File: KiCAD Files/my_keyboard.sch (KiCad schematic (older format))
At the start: 47 parts, among them K1 KEYSW, K10 KEYSW, K11 KEYSW, K12 KEYSW, K13 KEYSW, K14 KEYSW, K15 KEYSW, K16 KEYSW, K17 KEYSW, K2 KEYSW, K3 KEYSW, K4 KEYSW, K5 KEYSW, K6 KEYSW, K7 KEYSW, K8 KEYSW, K9 KEYSW, SW1 SW_Push, SW2 Rotary_Encoder_Switch, SW3 Rotary_Encoder_Switch, SW4 Rotary_Encoder_Switch

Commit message: Update PCB
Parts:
- D1, D10, D11, D12, D13, D14, D15, D16, D17, D18, D19, D2, D20, D3, D4, D5, D6, D7, D8, D9: footprint Diode_THT:D_DO-35_SOD27_P10.16mm_Horizontal -> keyboard_parts:D_SOD123_axial
- H1, H2, H3, H4: footprint (none) -> MountingHole:MountingHole_4.3mm_M4_Pad_Via
- SW1: footprint Button_Switch_THT:SW_PUSH_6mm -> Button_Switch_SMD:SW_PUSH_4_5.1x5.1mm
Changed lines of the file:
@@
 F 0 "D1" V 6954 1628 50  0000 L CNN
 F 1 "DIODE" V 7045 1628 50  0000 L CNN
-F 2 "Diode_THT:D_DO-35_SOD27_P10.16mm_Horizontal" H 7000 1500 50  0001 C CNN
+F 2 "keyboard_parts:D_SOD123_axial" H 7000 1500 50  0001 C CNN
 F 3 "~" H 7000 1500 50  0001 C CNN
 	1    7000 1500
@@
 F 0 "D2" V 6954 2478 50  0000 L CNN
 F 1 "DIODE" V 7045 2478 50  0000 L CNN
-F 2 "Diode_THT:D_DO-35_SOD27_P10.16mm_Horizontal" H 7000 2350 50  0001 C CNN
+F 2 "keyboard_parts:D_SOD123_axial" H 7000 2350 50  0001 C CNN
 F 3 "~" H 7000 2350 50  0001 C CNN
 	1    7000 2350
@@
 F 0 "D3" V 6954 3328 50  0000 L CNN
 F 1 "DIODE" V 7045 3328 50  0000 L CNN
-F 2 "Diode_THT:D_DO-35_SOD27_P10.16mm_Horizontal" H 7000 3200 50  0001 C CNN
+F 2 "keyboard_parts:D_SOD123_axial" H 7000 3200 50  0001 C CNN
 F 3 "~" H 7000 3200 50  0001 C CNN
 	1    7000 3200
@@
 F 0 "D4" V 6954 4178 50  0000 L CNN
 F 1 "DIODE" V 7045 4178 50  0000 L CNN
-F 2 "Diode_THT:D_DO-35_SOD27_P10.16mm_Horizontal" H 7000 4050 50  0001 C CNN
+F 2 "keyboard_parts:D_SOD123_axial" H 7000 4050 50  0001 C CNN
 F 3 "~" H 7000 4050 50  0001 C CNN
 	1    7000 4050
@@
 F 0 "D5" V 6954 5028 50  0000 L CNN
 F 1 "DIODE" V 7045 5028 50  0000 L CNN
-F 2 "Diode_THT:D_DO-35_SOD27_P10.16mm_Horizontal" H 7000 4900 50  0001 C CNN
+F 2 "keyboard_parts:D_SOD123_axial" H 7000 4900 50  0001 C CNN
 F 3 "~" H 7000 4900 50  0001 C CNN
 	1    7000 4900
@@
 F 0 "D6" V 7954 1628 50  0000 L CNN
 F 1 "DIODE" V 8045 1628 50  0000 L CNN
-F 2 "Diode_THT:D_DO-35_SOD27_P10.16mm_Horizontal" H 8000 1500 50  0001 C CNN
+F 2 "keyboard_parts:D_SOD123_axial" H 8000 1500 50  0001 C CNN
 F 3 "~" H 8000 1500 50  0001 C CNN
 	1    8000 1500
@@
 F 0 "D7" V 7954 2478 50  0000 L CNN
 F 1 "DIODE" V 8045 2478 50  0000 L CNN
-F 2 "Diode_THT:D_DO-35_SOD27_P10.16mm_Horizontal" H 8000 2350 50  0001 C CNN
+F 2 "keyboard_parts:D_SOD123_axial" H 8000 2350 50  0001 C CNN
 F 3 "~" H 8000 2350 50  0001 C CNN
 	1    8000 2350
@@
 F 0 "D8" V 7954 3328 50  0000 L CNN
 F 1 "DIODE" V 8045 3328 50  0000 L CNN
-F 2 "Diode_THT:D_DO-35_SOD27_P10.16mm_Horizontal" H 8000 3200 50  0001 C CNN
+F 2 "keyboard_parts:D_SOD123_axial" H 8000 3200 50  0001 C CNN
 F 3 "~" H 8000 3200 50  0001 C CNN
 	1    8000 3200
@@
 F 0 "D9" V 7954 4178 50  0000 L CNN
 F 1 "DIODE" V 8045 4178 50  0000 L CNN
-F 2 "Diode_THT:D_DO-35_SOD27_P10.16mm_Horizontal" H 8000 4050 50  0001 C CNN
+F 2 "keyboard_parts:D_SOD123_axial" H 8000 4050 50  0001 C CNN
 F 3 "~" H 8000 4050 50  0001 C CNN
 	1    8000 4050
@@
 F 0 "D10" V 7954 5028 50  0000 L CNN
 F 1 "DIODE" V 8045 5028 50  0000 L CNN
-F 2 "Diode_THT:D_DO-35_SOD27_P10.16mm_Horizontal" H 8000 4900 50  0001 C CNN
+F 2 "keyboard_parts:D_SOD123_axial" H 8000 4900 50  0001 C CNN
 F 3 "~" H 8000 4900 50  0001 C CNN
 	1    8000 4900
@@
 F 0 "D11" V 8954 1628 50  0000 L CNN
 F 1 "DIODE" V 9045 1628 50  0000 L CNN
-F 2 "Diode_THT:D_DO-35_SOD27_P10.16mm_Horizontal" H 9000 1500 50  0001 C CNN
+F 2 "keyboard_parts:D_SOD123_axial" H 9000 1500 50  0001 C CNN
 F 3 "~" H 9000 1500 50  0001 C CNN
 	1    9000 1500
@@
 F 0 "D12" V 8954 2478 50  0000 L CNN
 F 1 "DIODE" V 9045 2478 50  0000 L CNN
-F 2 "Diode_THT:D_DO-35_SOD27_P10.16mm_Horizontal" H 9000 2350 50  0001 C CNN
+F 2 "keyboard_parts:D_SOD123_axial" H 9000 2350 50  0001 C CNN
 F 3 "~" H 9000 2350 50  0001 C CNN
 	1    9000 2350
@@
 F 0 "D13" V 8954 3328 50  0000 L CNN
 F 1 "DIODE" V 9045 3328 50  0000 L CNN
-F 2 "Diode_THT:D_DO-35_SOD27_P10.16mm_Horizontal" H 9000 3200 50  0001 C CNN
+F 2 "keyboard_parts:D_SOD123_axial" H 9000 3200 50  0001 C CNN
 F 3 "~" H 9000 3200 50  0001 C CNN
 	1    9000 3200
@@
 F 0 "D14" V 8954 4178 50  0000 L CNN
 F 1 "DIODE" V 9045 4178 50  0000 L CNN
-F 2 "Diode_THT:D_DO-35_SOD27_P10.16mm_Horizontal" H 9000 4050 50  0001 C CNN
+F 2 "keyboard_parts:D_SOD123_axial" H 9000 4050 50  0001 C CNN
 F 3 "~" H 9000 4050 50  0001 C CNN
 	1    9000 4050
@@
 F 0 "D18" V 9954 3328 50  0000 L CNN
 F 1 "DIODE" V 10045 3328 50  0000 L CNN
-F 2 "Diode_THT:D_DO-35_SOD27_P10.16mm_Horizontal" H 10000 3200 50  0001 C CNN
+F 2 "keyboard_parts:D_SOD123_axial" H 10000 3200 50  0001 C CNN
 F 3 "~" H 10000 3200 50  0001 C CNN
 	1    10000 3200
@@
 F 0 "D16" V 9954 1628 50  0000 L CNN
 F 1 "DIODE" V 10045 1628 50  0000 L CNN
-F 2 "Diode_THT:D_DO-35_SOD27_P10.16mm_Horizontal" H 10000 1500 50  0001 C CNN
+F 2 "keyboard_parts:D_SOD123_axial" H 10000 1500 50  0001 C CNN
 F 3 "~" H 10000 1500 50  0001 C CNN
 	1    10000 1500
@@
 F 0 "D17" V 9954 2478 50  0000 L CNN
 F 1 "DIODE" V 10045 2478 50  0000 L CNN
-F 2 "Diode_THT:D_DO-35_SOD27_P10.16mm_Horizontal" H 10000 2350 50  0001 C CNN
+F 2 "keyboard_parts:D_SOD123_axial" H 10000 2350 50  0001 C CNN
 F 3 "~" H 10000 2350 50  0001 C CNN
 	1    10000 2350
@@
 F 0 "D19" V 9954 4178 50  0000 L CNN
 F 1 "DIODE" V 10045 4178 50  0000 L CNN
-F 2 "Diode_THT:D_DO-35_SOD27_P10.16mm_Horizontal" H 10000 4050 50  0001 C CNN
+F 2 "keyboard_parts:D_SOD123_axial" H 10000 4050 50  0001 C CNN
 F 3 "~" H 10000 4050 50  0001 C CNN
 	1    10000 4050
@@
 F 0 "SW1" H 1300 6835 50  0000 C CNN
 F 1 "SW_Push" H 1300 6744 50  0000 C CNN
-F 2 "Button_Switch_THT:SW_PUSH_6mm" H 1300 6750 50  0001 C CNN
+F 2 "Button_Switch_SMD:SW_PUSH_4_5.1x5.1mm" H 1300 6750 50  0001 C CNN
 F 3 "~" H 1300 6750 50  0001 C CNN
 	1    1300 6550
@@
 F 0 "D15" V 8954 5028 50  0000 L CNN
 F 1 "DIODE" V 9045 5028 50  0000 L CNN
-F 2 "Diode_THT:D_DO-35_SOD27_P10.16mm_Horizontal" H 9000 4900 50  0001 C CNN
+F 2 "keyboard_parts:D_SOD123_axial" H 9000 4900 50  0001 C CNN
 F 3 "~" H 9000 4900 50  0001 C CNN
 	1    9000 4900
@@
 F 0 "D20" V 9954 5028 50  0000 L CNN
 F 1 "DIODE" V 10045 5028 50  0000 L CNN
-F 2 "Diode_THT:D_DO-35_SOD27_P10.16mm_Horizontal" H 10000 4900 50  0001 C CNN
+F 2 "keyboard_parts:D_SOD123_axial" H 10000 4900 50  0001 C CNN
 F 3 "~" H 10000 4900 50  0001 C CNN
 	1    10000 4900
@@
 F 0 "H1" V 4604 4150 50  0000 L CNN
 F 1 "MountingHole_Pad" V 4695 4150 50  0000 L CNN
-F 2 "" H 4650 4000 50  0001 C CNN
+F 2 "MountingHole:MountingHole_4.3mm_M4_Pad_Via" H 4650 4000 50  0001 C CNN
 F 3 "~" H 4650 4000 50  0001 C CNN
 	1    4650 4000
@@
 F 0 "H2" V 4604 4450 50  0000 L CNN
 F 1 "MountingHole_Pad" V 4695 4450 50  0000 L CNN
-F 2 "" H 4650 4300 50  0001 C CNN
+F 2 "MountingHole:MountingHole_4.3mm_M4_Pad_Via" H 4650 4300 50  0001 C CNN
 F 3 "~" H 4650 4300 50  0001 C CNN
 	1    4650 4300
@@
 F 0 "H3" V 4604 4750 50  0000 L CNN
 F 1 "MountingHole_Pad" V 4695 4750 50  0000 L CNN
-F 2 "" H 4650 4600 50  0001 C CNN
+F 2 "MountingHole:MountingHole_4.3mm_M4_Pad_Via" H 4650 4600 50  0001 C CNN
 F 3 "~" H 4650 4600 50  0001 C CNN
 	1    4650 4600
@@
 F 0 "H4" V 4604 5050 50  0000 L CNN
 F 1 "MountingHole_Pad" V 4695 5050 50  0000 L CNN
-F 2 "" H 4650 4900 50  0001 C CNN
+F 2 "MountingHole:MountingHole_4.3mm_M4_Pad_Via" H 4650 4900 50  0001 C CNN
 F 3 "~" H 4650 4900 50  0001 C CNN
 	1    4650 4900

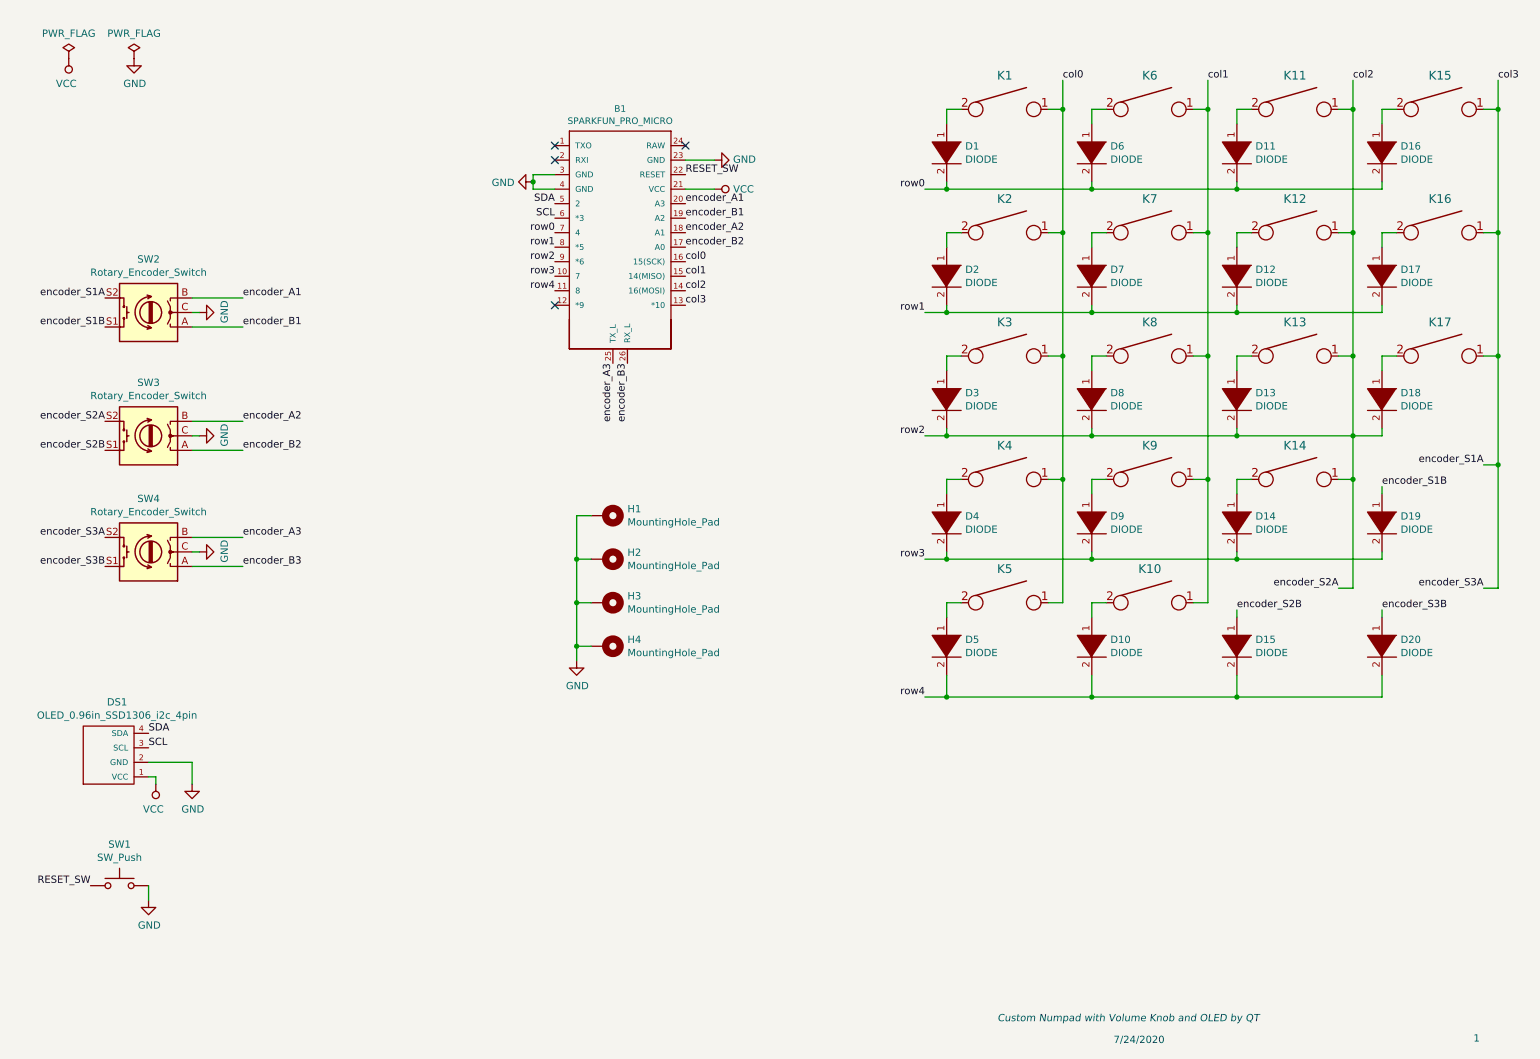
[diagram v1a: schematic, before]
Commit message: Updated KiCAD Schem
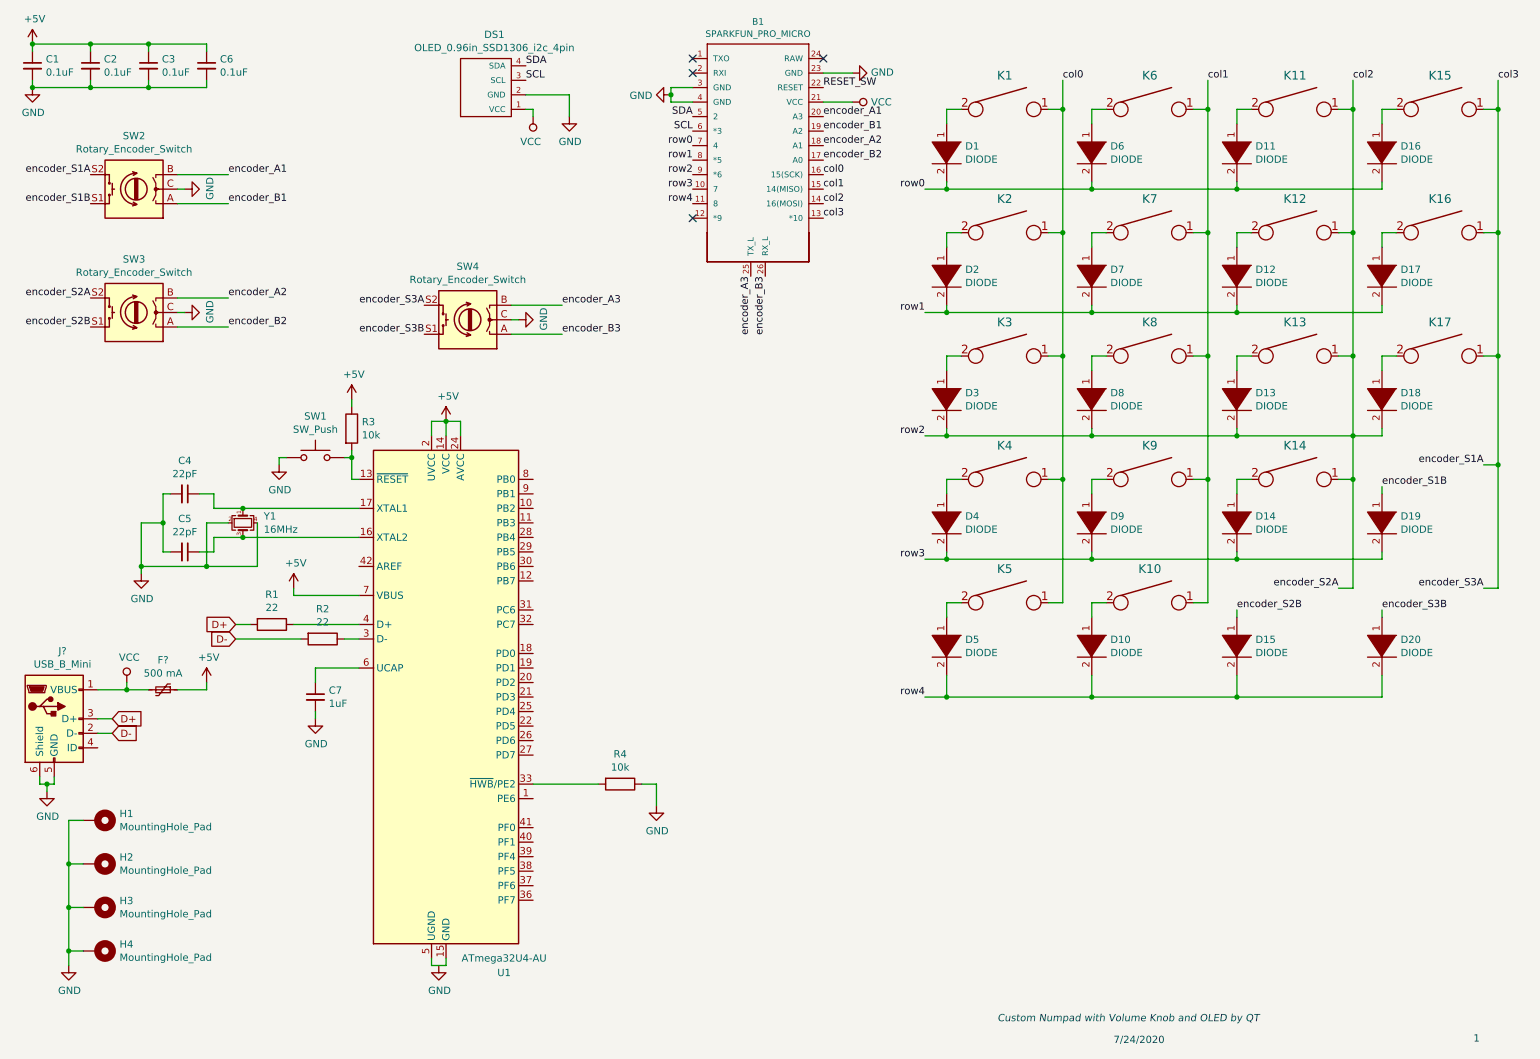
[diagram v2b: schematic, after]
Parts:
- added C1, C2, C3, C6: 0.1uF, symbol Device:C_Small
- added C4, C5: 22pF, symbol Device:C_Small
- added C7: 1uF, symbol Device:C_Small
- added F?: 500 mA, symbol Device:Polyfuse_Small
- added J?: USB_B_Mini, symbol Connector:USB_B_Mini
- added R1, R2: 22, symbol Device:R
- added R3, R4: 10k, symbol Device:R
- added U1: ATmega32U4-AU, Package_QFP:TQFP-44_10x10mm_P0.8mm, symbol MCU_Microchip_ATmega:ATmega32U4-AU
- added Y1: 16MHz, symbol Device:Crystal_GND24_Small
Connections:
- net GND: now also SW1.1, C1.2, C2.2, C3.2, C4.2, C5.2, C6.2, C7.2, J?.5 (GND), J?.6 (Shield), R4.1, Y1.2, Y1.4; no longer SW1.2
- net RESET_SW: no longer SW1.1
- net VCC: now also F?.2, J?.1 (VBUS)
- new net: R3.2, SW1.2, U1.13 (~RESET)
- new net: U1.15 (GND), U1.23 (GND), U1.35 (GND), U1.43 (GND), U1.5 (UGND)
- new net: C5.1, U1.16 (XTAL2), Y1.3
- new net: C4.1, U1.17 (XTAL1), Y1.1
- new net: R2.1, U1.3 (D-)
- new net: R4.2, U1.33 (~HWB~/PE2)
- new net: R1.1, U1.4 (D+)
- new net: C7.1, U1.6 (UCAP)
- new net +5V: C1.1, C2.1, C3.1, C6.1, F?.1, R3.1, U1.14 (VCC), U1.2 (UVCC), U1.24 (AVCC), U1.34 (VCC), U1.44 (AVCC), U1.7 (VBUS)
- new net D+: J?.3 (D+), R1.2
- new net D-: J?.2 (D-), R2.2
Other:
- moved on the sheet: B1, DS1, H1, H2, H3, H4, SW1, SW2, SW3, SW4
